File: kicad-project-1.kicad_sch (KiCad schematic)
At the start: 8 parts, among them U1 Pico-MCU_RaspberryPi_and_Boar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, U2 Pololu_4Ch

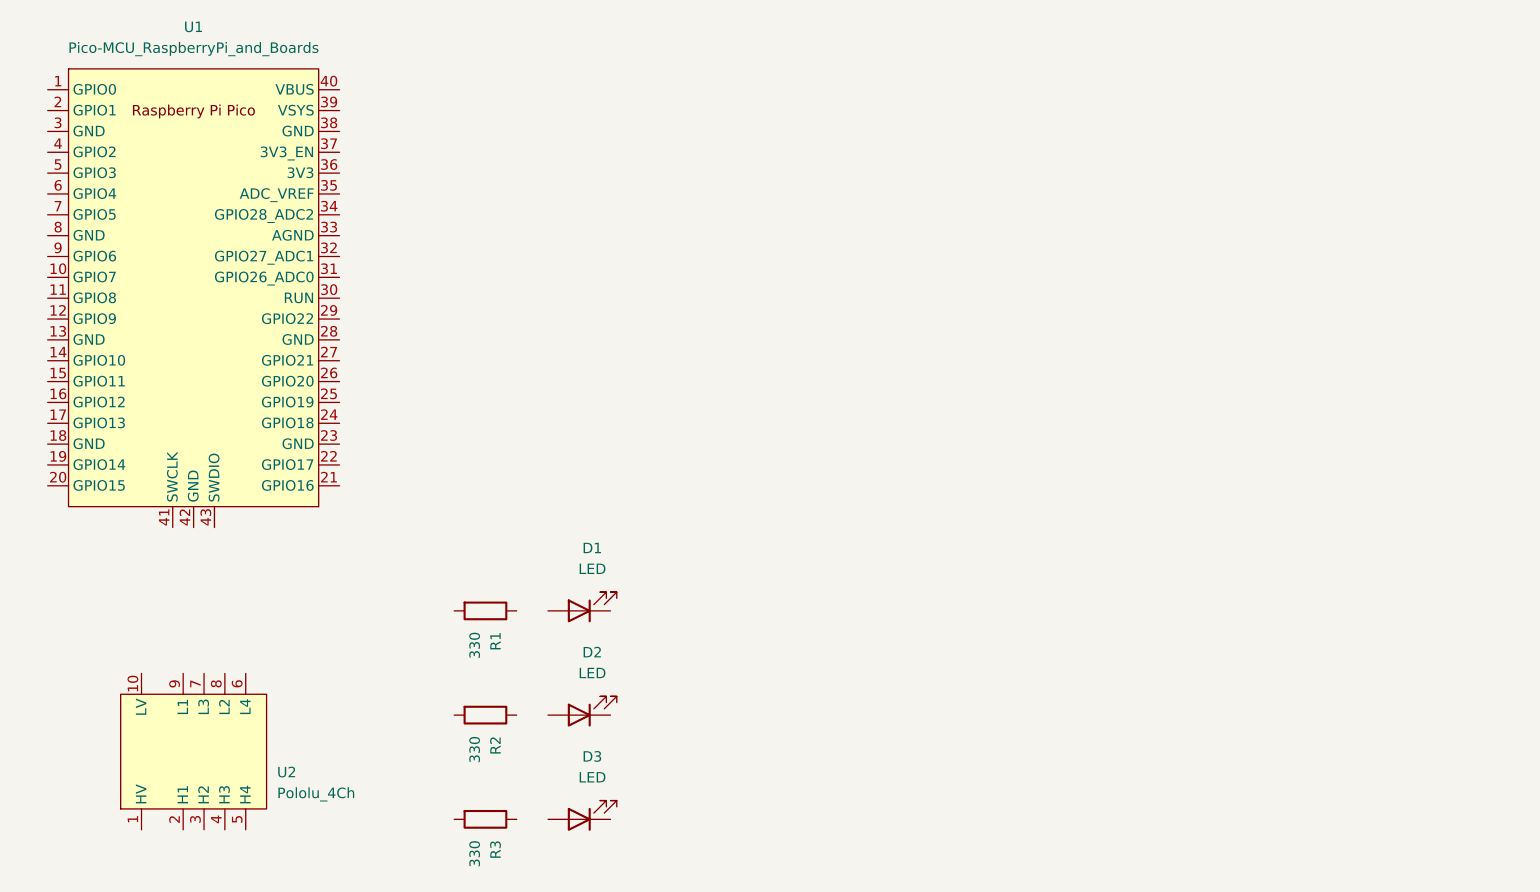
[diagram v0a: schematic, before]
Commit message: testing
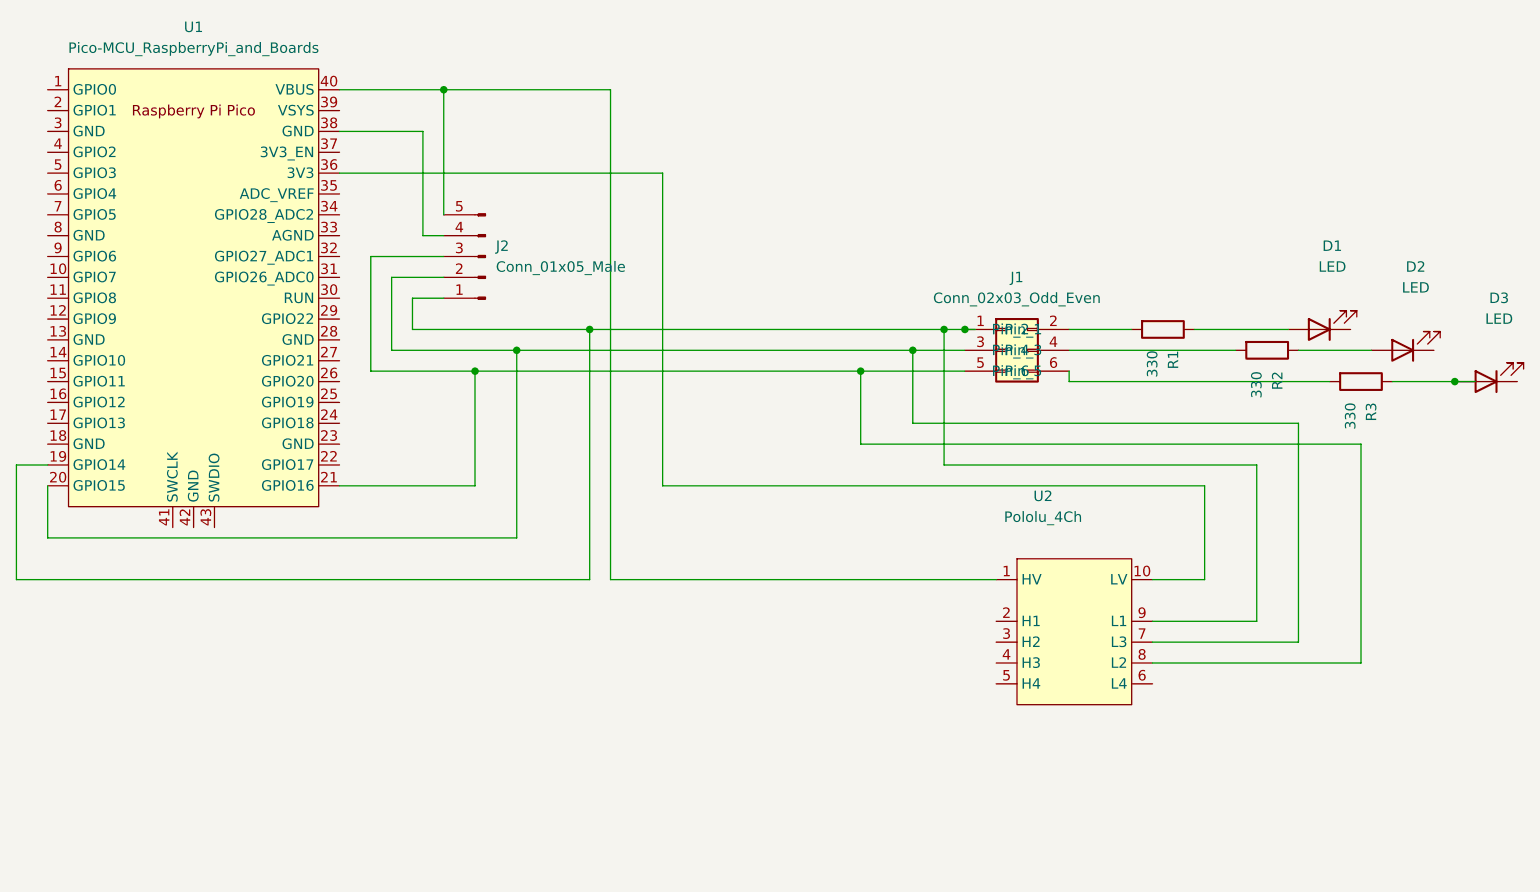
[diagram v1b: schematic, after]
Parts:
- added J1: Conn_02x03_Odd_Even, Connector_PinSocket_2.00mm:PinSocket_2x03_P2.00mm_Horizontal, symbol Connector_Generic:Conn_02x03_Odd_Even
- added J2: Conn_01x05_Male, Connector_PinSocket_1.00mm:PinSocket_1x05_P1.00mm_Vertical, symbol Connector:Conn_01x05_Male
- D1, D2, D3: footprint (none) -> LED_THT:LED_D3.0mm
- R1, R2, R3: footprint (none) -> Resistor_SMD:R_0201_0603Metric
- U1: footprint RPi_Pico:RPi_Pico_SMD_TH -> Package_DIP:DIP-40_W25.4mm_Socket_LongPads
- U2: footprint (none) -> Package_DIP:DIP-10_W7.62mm
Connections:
- net at R3.1: now also D3.2 (A)
- net at R3.2: now also J1.6 (Pin_6)
- net at R1.1: now also D1.2 (A)
- net at R1.2: now also J1.2 (Pin_2)
- net at U1.19 (GPIO14): now also U2.9 (L1), J1.1 (Pin_1), J2.1 (Pin_1)
- net at U1.20 (GPIO15): now also U2.7 (L3), J1.3 (Pin_3), J2.2 (Pin_2)
- net at U1.21 (GPIO16): now also U2.8 (L2), J1.5 (Pin_5), J2.3 (Pin_3)
- net at U1.36 (3V3): now also U2.10 (LV)
- net at U1.38 (GND): now also J2.4 (Pin_4)
- net at U1.40 (VBUS): now also U2.1 (HV), J2.5 (Pin_5)
- net at R2.1: now also D2.2 (A)
- net at R2.2: now also J1.4 (Pin_4)
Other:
- moved on the sheet: D1, R1, R2, R3, U2
